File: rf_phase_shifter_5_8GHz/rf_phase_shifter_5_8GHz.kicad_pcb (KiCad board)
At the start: 2 copper layers, 12 parts, among them J1 Conn_Coaxial, J2 Conn_Coaxial, J3 Conn_Coaxial

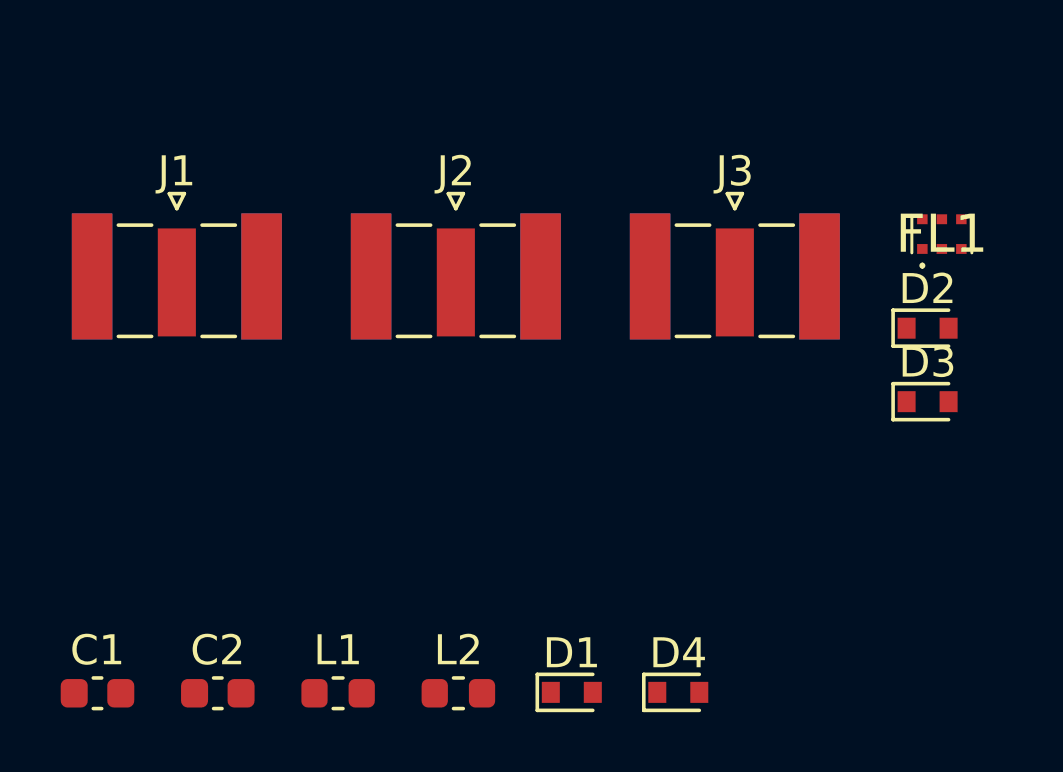
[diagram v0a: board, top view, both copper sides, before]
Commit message: update
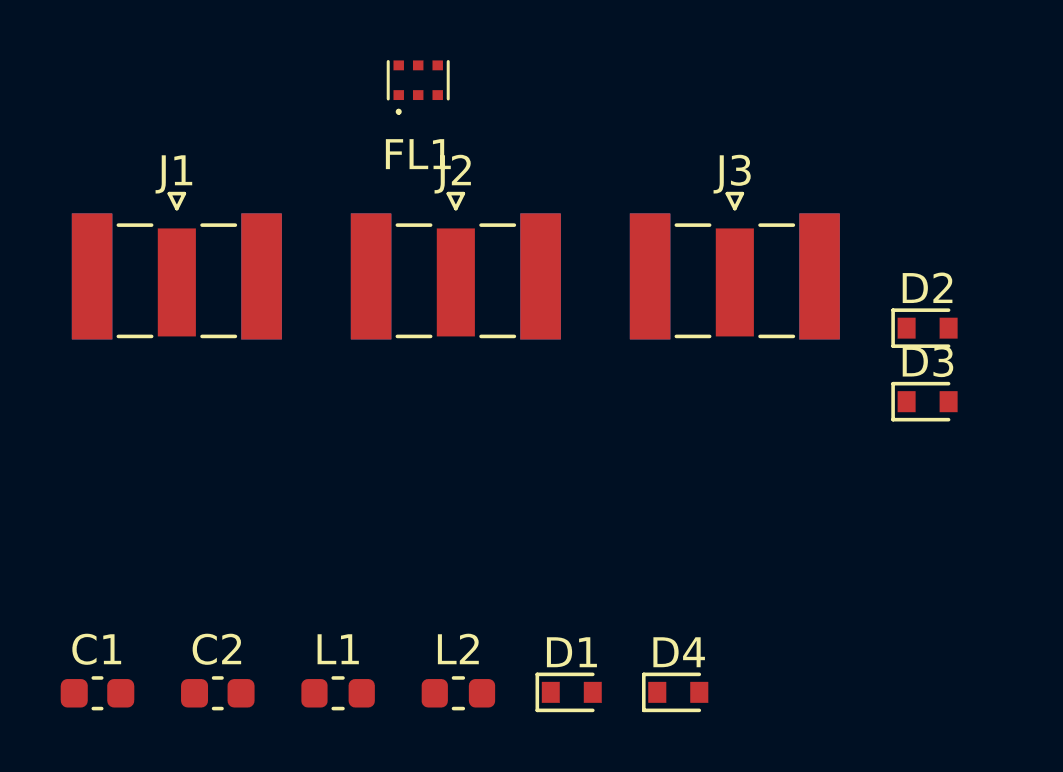
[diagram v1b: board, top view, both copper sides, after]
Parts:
- FL1: value C2327J5003AHF -> C5060J5003AHF; footprint RF:C2327J5003AHF -> analog_rf_phase_shifter_module:C5060J5003AHF
- moved FL1 18.2 mm to (36.3, 15.9)
